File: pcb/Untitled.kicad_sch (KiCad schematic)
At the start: 57 parts, among them J1 Conn_01x08_Socket, J2 Micro_SD_Card_Det1, J3 USB_C_Receptacle_USB2.0_14P, J4 Conn_01x02, J5 Conn_Coaxial, Q1 FS8205A, Q2 AO3407A, SW1 reset, SW10 SW_Push, SW2 boot, SW3 SW_Push, SW4 SW_Push, SW5 SW_Push, SW6 SW_Push, SW7 SW_Push, SW8 SW_Push, SW9 SW_Push, U1 ESP32-S3-WROOM-1, U10 RV-3028-C8-32.768KHZ-1PPM-TA-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, U11 BMP390, U2 MAX-M10S, U3 USBLC6-2SC6, U4 MCP73831-2-MC, U5 AP2112K-3.3, U6 DW01A, U7 LIS3MDL, U9 SHT4x

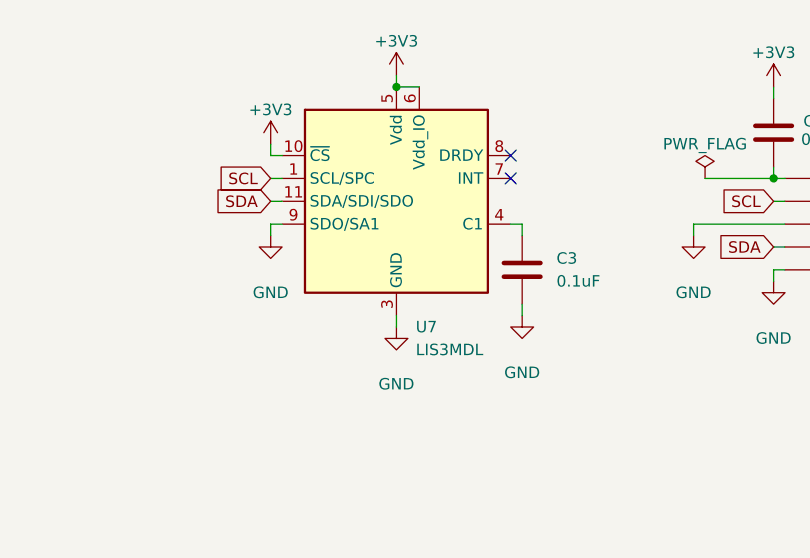
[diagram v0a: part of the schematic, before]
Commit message: update
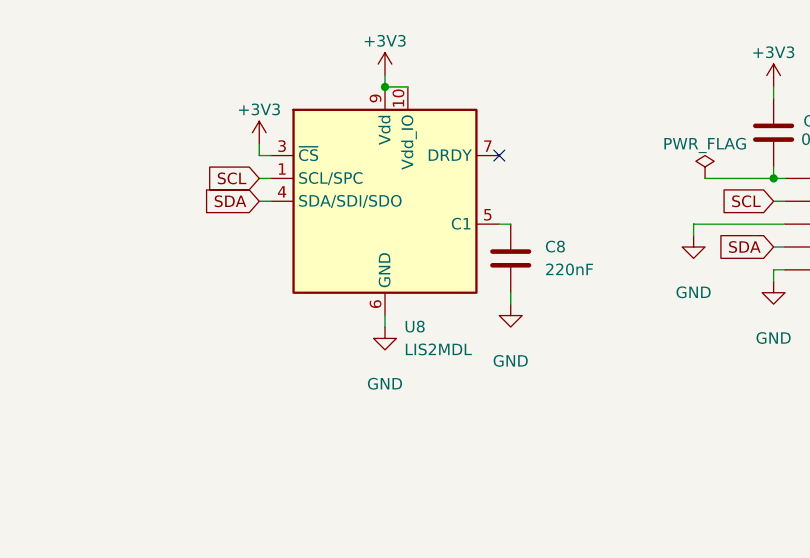
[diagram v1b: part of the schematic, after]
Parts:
- removed C3: 0.1uF, Capacitor_SMD:C_0402_1005Metric, symbol Device:C
- removed U7: LIS3MDL, Package_LGA:LGA-12_2x2mm_P0.5mm, symbol Sensor_Magnetic:LIS3MDL
- added C8: 220nF, Capacitor_SMD:C_0402_1005Metric, symbol Device:C
- added U8: LIS2MDL, Package_LGA:LGA-12_2x2mm_P0.5mm, symbol Sensor_Magnetic:LIS2MDL
- Q1: footprint FS8205A:SOP65P640X120-8N -> Package_TO_SOT_SMD:SOT-23-6
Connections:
- net +3V3: now also U8.10 (Vdd_IO), U8.3 (~{CS}), U8.9 (Vdd)
- net GND: now also C8.2, U8.6 (GND), U8.8 (GND)
- net SCL: now also U8.1 (SCL/SPC)
- net SDA: now also U8.4 (SDA/SDI/SDO)
- new net: C8.1, U8.5 (C1)
- no-connect marks 24 -> 23
